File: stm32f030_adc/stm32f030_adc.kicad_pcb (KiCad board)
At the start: 2 copper layers, 43 parts, among them Q1 BC337, U1 STM32F103C6Tx, U2 AMS1117-3.3, X1 USB_B_Micro, Y2 8 MHz

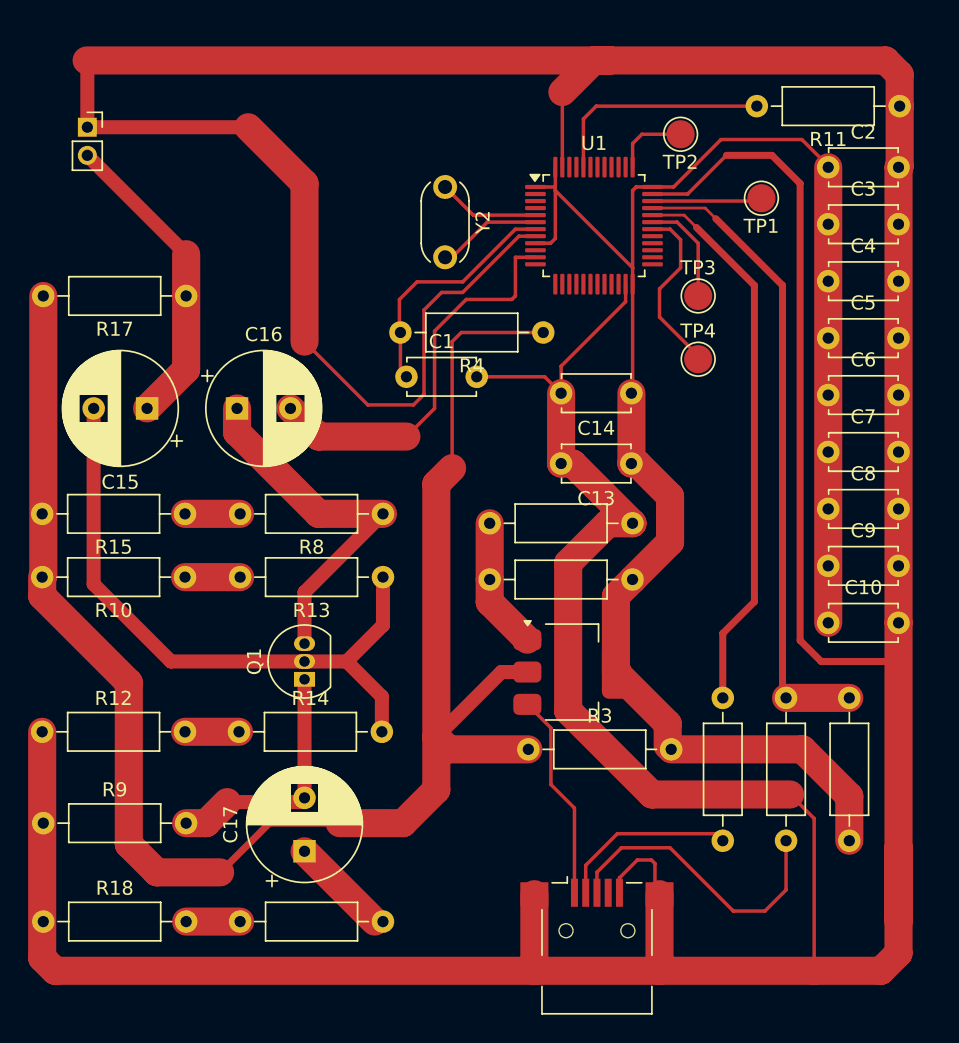
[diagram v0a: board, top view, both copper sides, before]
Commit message: Dimensions: narrower
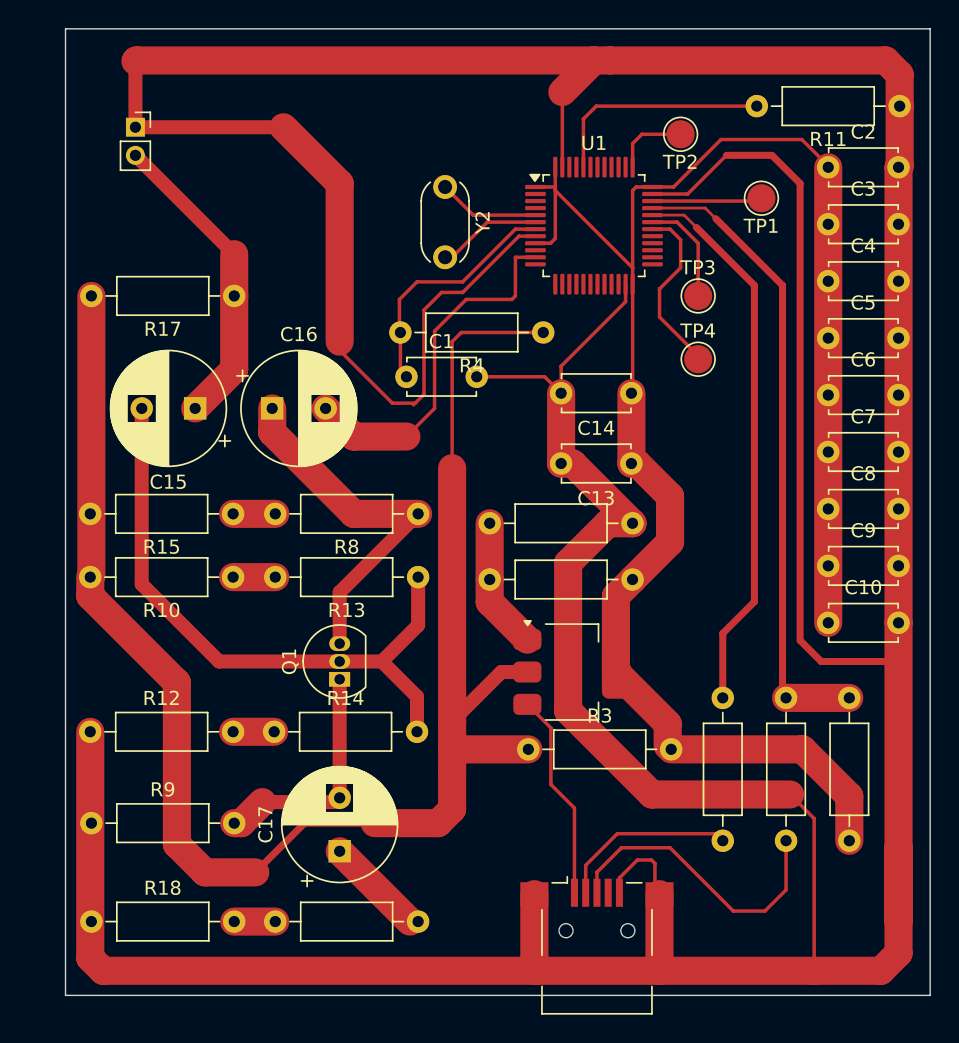
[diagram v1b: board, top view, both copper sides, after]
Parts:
- moved C15 3.42 mm to (125.2, 105.5)
- moved MK1 3.42 mm to (121.0, 85.5)
- moved R10 3.42 mm to (127.9, 117.5)
- moved R12 3.42 mm to (117.8, 128.5)
- moved R15 3.42 mm to (127.9, 113.0)
- moved R17 3.42 mm to (128.0, 97.5)
- moved R18 3.42 mm to (117.8, 142.0)
- moved R9 3.42 mm to (117.8, 135.0)
- moved C16 2.50 mm to (130.7, 105.5)
- moved C17 2.50 mm to (135.5, 137.0)
- moved Q1 2.50 mm to (135.5, 124.8)
- moved R13 2.50 mm to (141.1, 117.5)
- moved R14 2.50 mm to (130.8, 128.5)
- moved R16 2.50 mm to (130.9, 142.0)
- moved R8 2.50 mm to (141.1, 113.0)
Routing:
- net GNDREF: track 419.0 -> 408.0 mm
- net +3V3: track 246.9 -> 241.9 mm
- net /Electret AMP/MIC_AMP_OUT: track 28.4 -> 25.9 mm
- net Net-(R16-Pad1): track 3.84 -> 2.92 mm
- net Net-(R15-Pad1): track 3.92 -> 3.00 mm
- net Net-(R12-Pad2): track 3.84 -> 2.92 mm
- net Net-(R10-Pad1): track 3.92 -> 3.00 mm
- net Net-(Q1-E): track 17.6 -> 16.7 mm
- net Net-(Q1-B): track 45.9 -> 45.0 mm
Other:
- board outline added: 61.5 x 68.8 mm
